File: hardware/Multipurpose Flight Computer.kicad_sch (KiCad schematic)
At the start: 82 parts, among them J1 Screw_Terminal_01x02, J2 Conn_01x03, J3 Conn_01x03, SW1 TS-1088-AR02016, SW2 TS-1088-AR02016, U1 BQ25883RGER, U2 ICM-45686, U3 STM32F722RETx, U4 BMP580, U5 TPS63070RNMR, U6 LMR51430, X1 X322525MOB4SI, X2 Q13FC1350000400

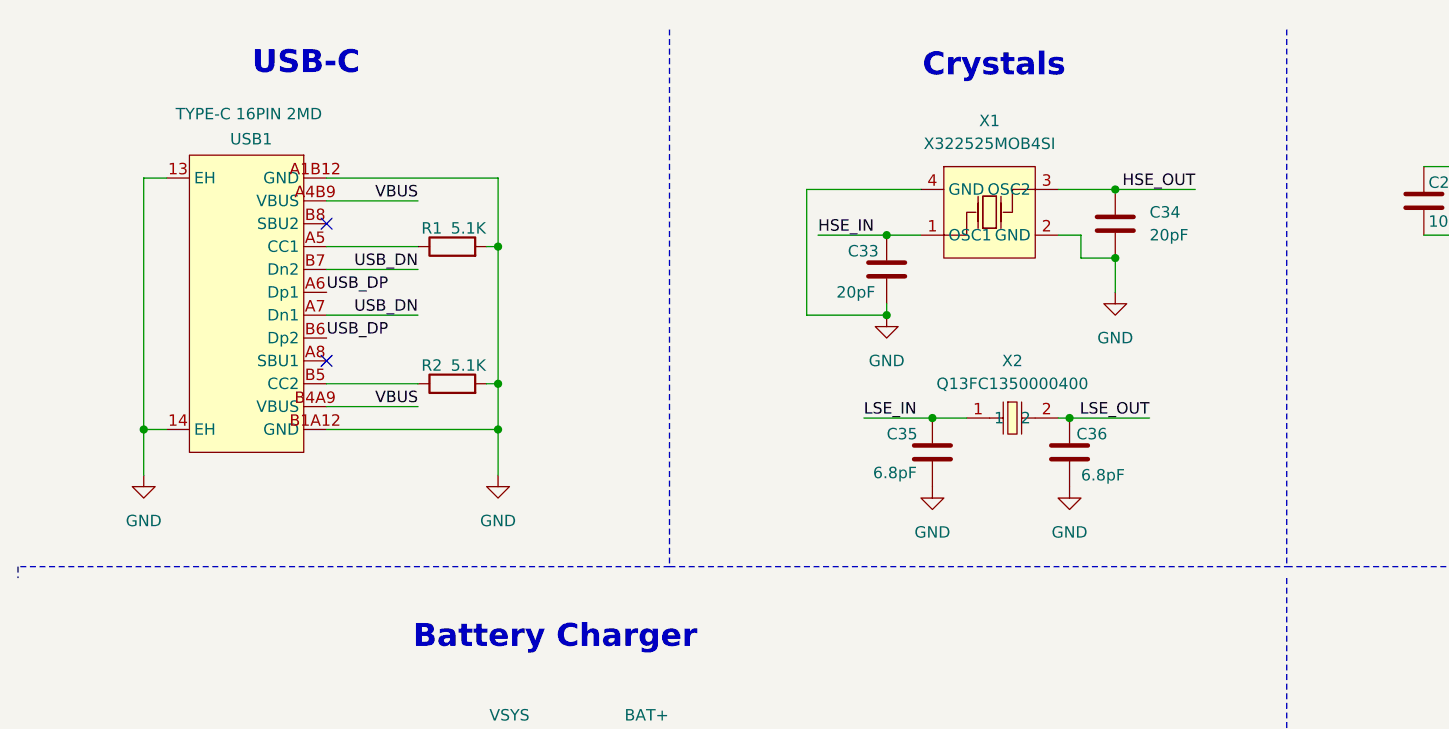
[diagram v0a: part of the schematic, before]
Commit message: Finalized Board Design
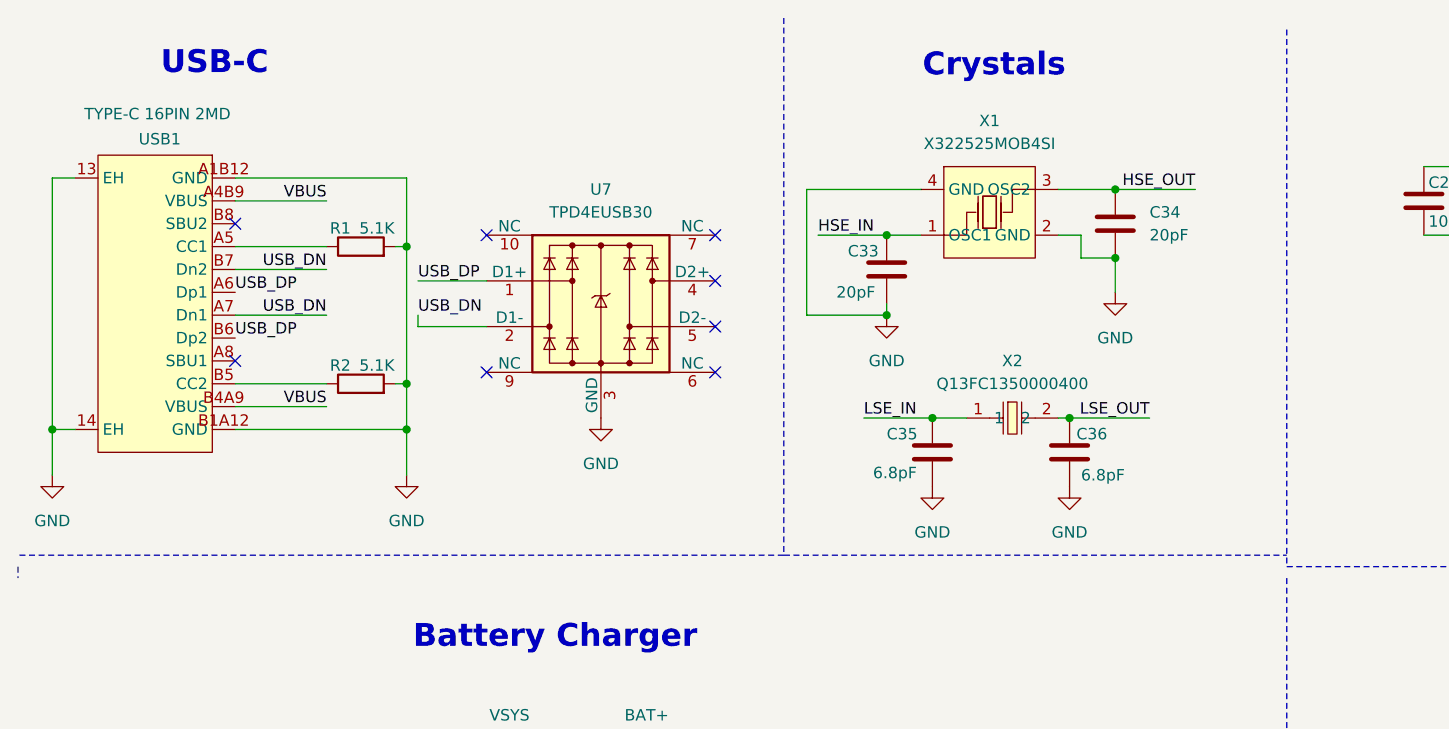
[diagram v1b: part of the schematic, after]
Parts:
- added U7: TPD4EUSB30, Package_SON:USON-10_2.5x1.0mm_P0.5mm, symbol Power_Protection:TPD4EUSB30
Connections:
- net GND: now also U7.3 (GND), U7.8 (GND)
- net USB_DN: now also U7.2 (D1-)
- net USB_DP: now also U7.1 (D1+)
- no-connect marks 32 -> 38
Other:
- moved on the sheet: R1, R2, USB1
